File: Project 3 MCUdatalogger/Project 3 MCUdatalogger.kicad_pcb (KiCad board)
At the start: 2 copper layers, 53.3 x 38.1 mm, 29 parts, among them J1 Conn_01x04_Pin, J2 Conn_01x09_Pin, J3 Conn_01x04_Pin, J4 Conn_02x03_Odd_Even, U1 24LC1025, U2 DS1337S_, U3 24LC1025, U4 ATMEGA328P-AU, Y1 32.768 KHz, Y2 16 MHz

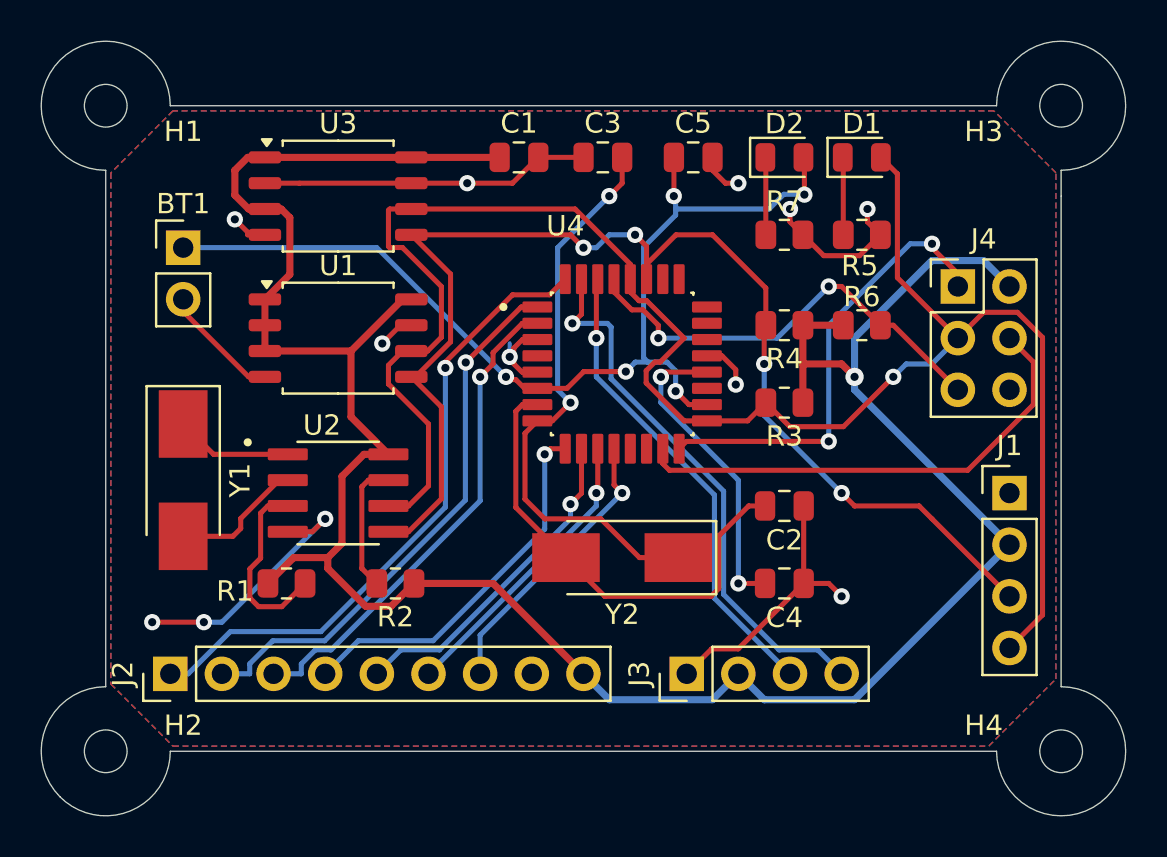
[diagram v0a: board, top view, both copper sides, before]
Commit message: Fixed outstanding issues
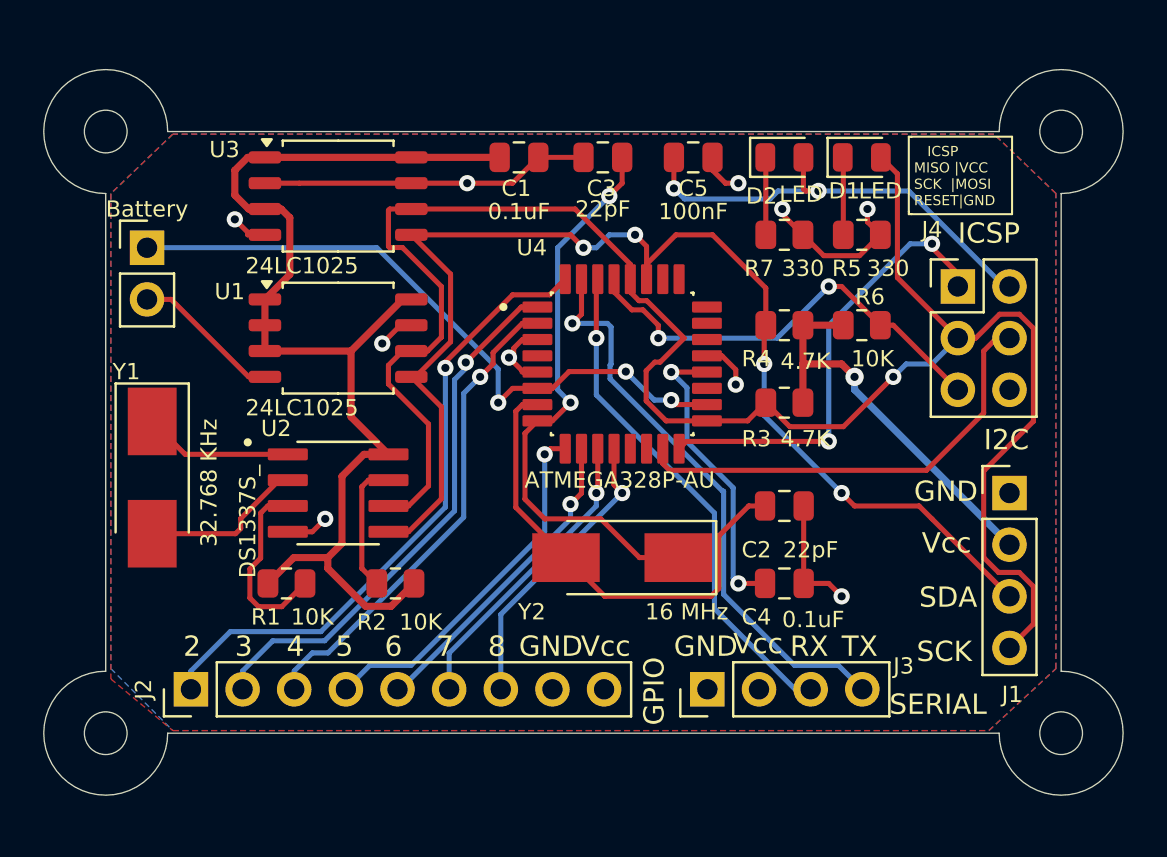
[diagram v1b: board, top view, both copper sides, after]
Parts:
- moved BT1 1.78 mm to (40.1, 64.1)
- moved Y1 1.53 mm to (40.4, 75.4)
- moved J3 1.27 mm to (67.7, 85.9)
- moved H1 1.27 mm to (38.1, 58.4)
- moved H3 1.27 mm to (85.1, 58.4)
- moved J2 1.27 mm to (42.3, 85.9)
- moved H2 0.89 mm to (38.1, 88.0)
- moved H4 0.89 mm to (85.1, 88.0)
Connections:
- BT1 pad 1: Net-(BT1-+) -> /Vcc
- C5 pad 1: Net-(BT1-+) -> /Vcc
- D2 pad 2: Net-(BT1-+) -> /Vcc
- U4 pad 18: Net-(BT1-+) -> /Vcc
- U4 pad 6: Net-(BT1-+) -> /Vcc
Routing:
- net Net-(BT1-+): track 50.0 -> 0.00 mm, vias 5 -> 0
- net GND: track 68.7 -> 52.4 mm, vias 12 -> 10
- net /Vcc: track 122.9 -> 131.4 mm, vias 1 -> 6
- net /SCK: track 91.5 -> 94.2 mm
- net /MOSI: track 24.2 -> 22.4 mm
- net /RX: track 23.4 -> 25.0 mm
- net Net-(U2-X1): track 5.76 -> 7.34 mm
- net Net-(U2-X2): track 6.58 -> 8.05 mm
- net /TX: track 27.3 -> 28.7 mm
- net /D6: track 16.4 -> 15.7 mm
- net /D5: track 18.5 -> 17.9 mm
- net Net-(U4-AREF): track 15.4 -> 14.8 mm
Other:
- board size 53.3 x 38.1 mm -> 53.1 x 35.7 mm
- board text added: "2"
- board text added: "3"
- board text added: "4"
- board text added: "5"
- board text added: "6"
- board text added: "7"
- board text added: "8"
- board text added: "GND"
- board text added: "GPIO"
- board text added: "I2C"
- board text added: "ICSP"
- board text added: "ICSP MISO |VCC SCK |MOSI RESET|GND"
- board text added: "RX"
- board text added: "SCK"
- board text added: "SDA"
- board text added: "SERIAL"
- board text added: "TX"
- board text added: "Vcc"
